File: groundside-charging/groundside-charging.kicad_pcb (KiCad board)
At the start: 2 copper layers, 45.7 x 71.1 mm, 29 parts, among them J1 12V In, J2 Charge Current Out (to Rocket), J3 Charge Voltage Sensing, Q1 SI4840BDY-T1-GE3, U1 LM317DCYR, U2 LM3478MA

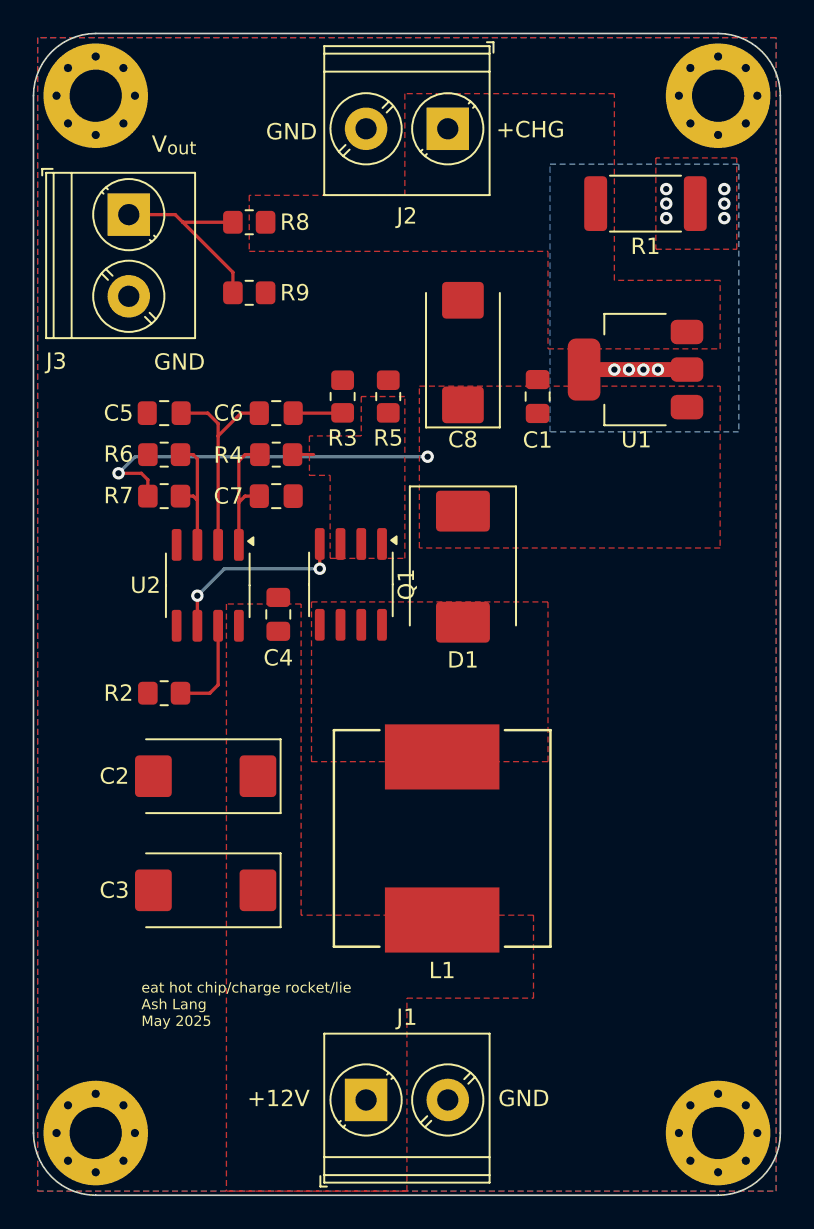
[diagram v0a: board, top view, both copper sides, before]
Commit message: generate gerbs, pdf
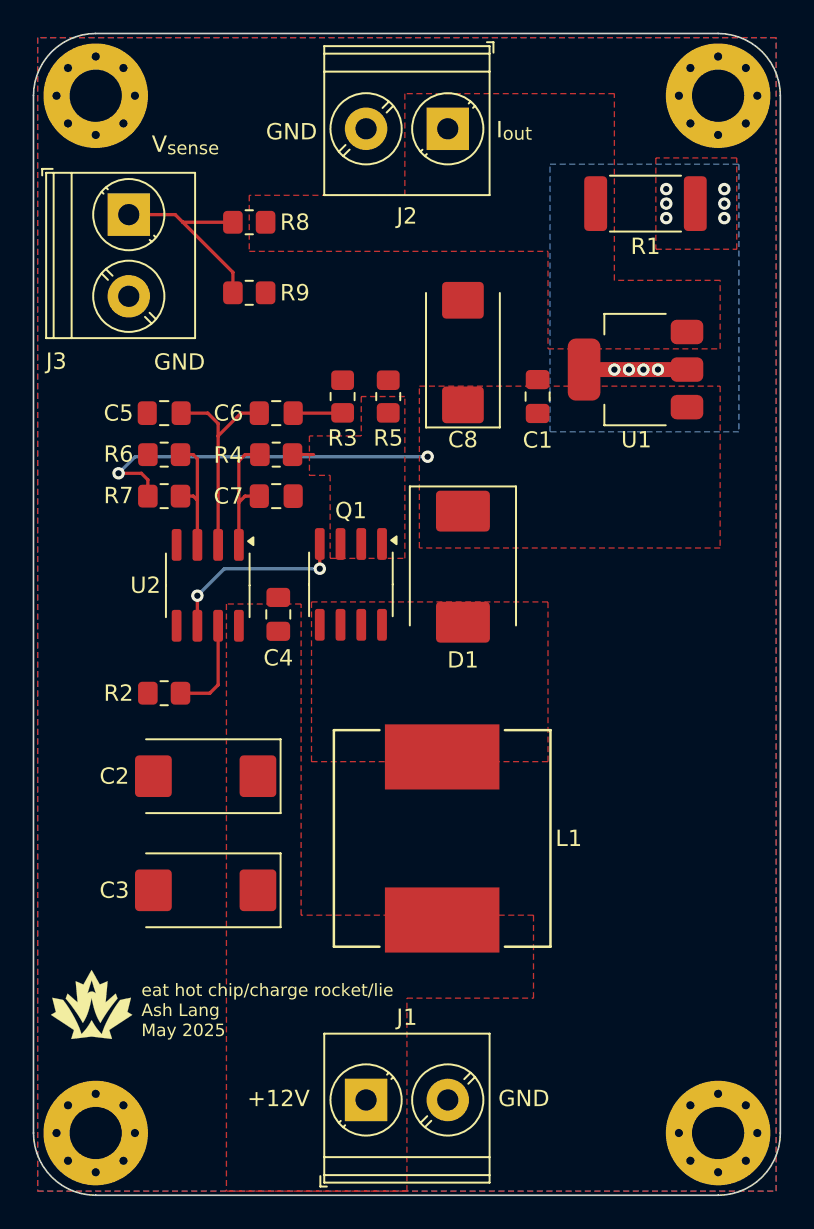
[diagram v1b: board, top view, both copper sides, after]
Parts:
- added G***: LOGO, groundside-charging:Logo_SilkScreen_5mm, F.Cu at (68.8, 151.6)
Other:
- board text added: "I_{out}"
- board text added: "V_{sense}"
- board text removed: "+CHG"
- board text removed: "V_{out}"
